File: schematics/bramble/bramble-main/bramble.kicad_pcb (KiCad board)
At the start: 2 copper layers, 50.4 x 70.6 mm, 78 parts, among them IC1 RP2040_QFN56, J1 Conn_01x05_Pin, J2 Conn_01x03_Pin, J3 Conn_01x03, J4 USB_C_Receptacle_USB2.0_16P, J5 U.FL, J6 Conn_02x06_Odd_Even, Q1 DMN3300U, Q2 FDN360P, SW1 STM_RESET, SW2 BOOT, SW3 RESET, U1 Opamp_Quad, U2 STM32L031F6P6TR, U3 MCP1700x-120xxMB, U4 RFM95W-915S2, U5 W25Q16JVSS, U6 MT25QL01GBBB8ESF-0SIT, Y1 Crystal, Y2 Crystal

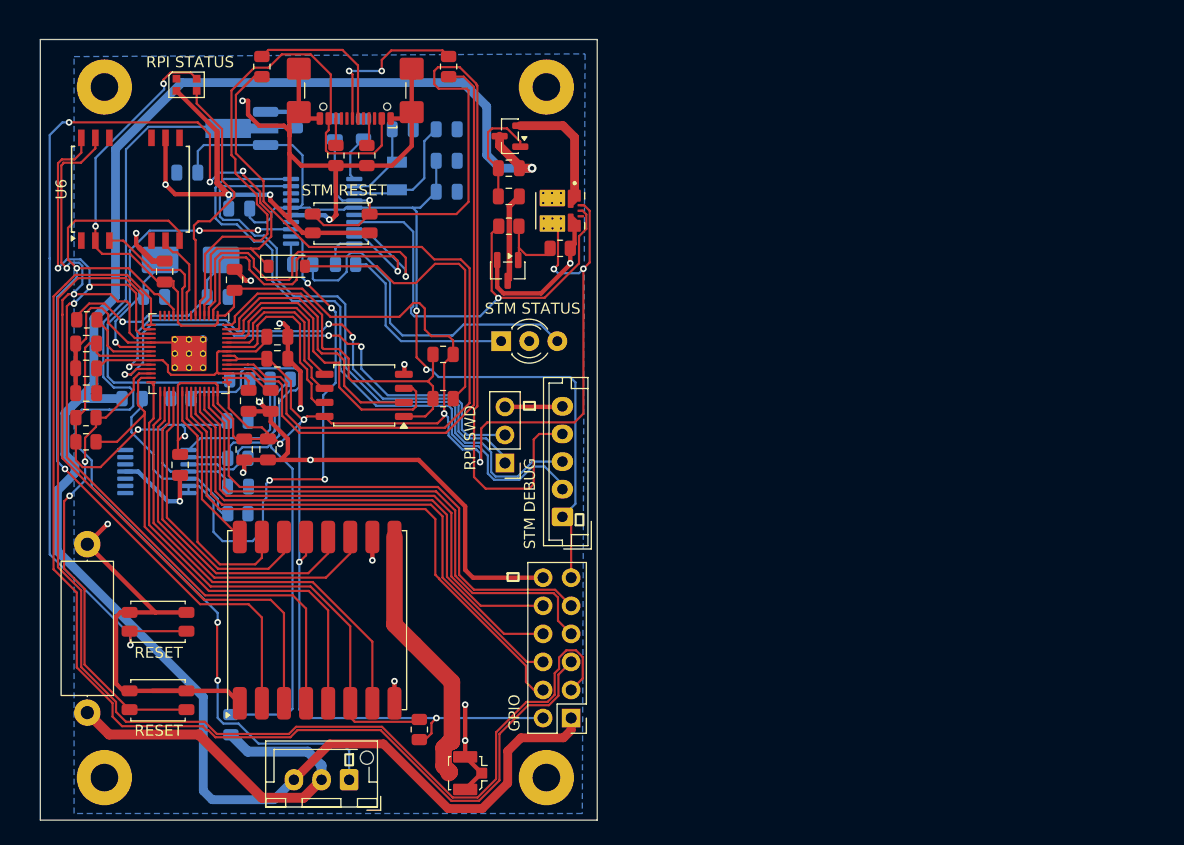
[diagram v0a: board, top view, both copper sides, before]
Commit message: Checking in v4 schematic/board prior to attempting jlcpcb run
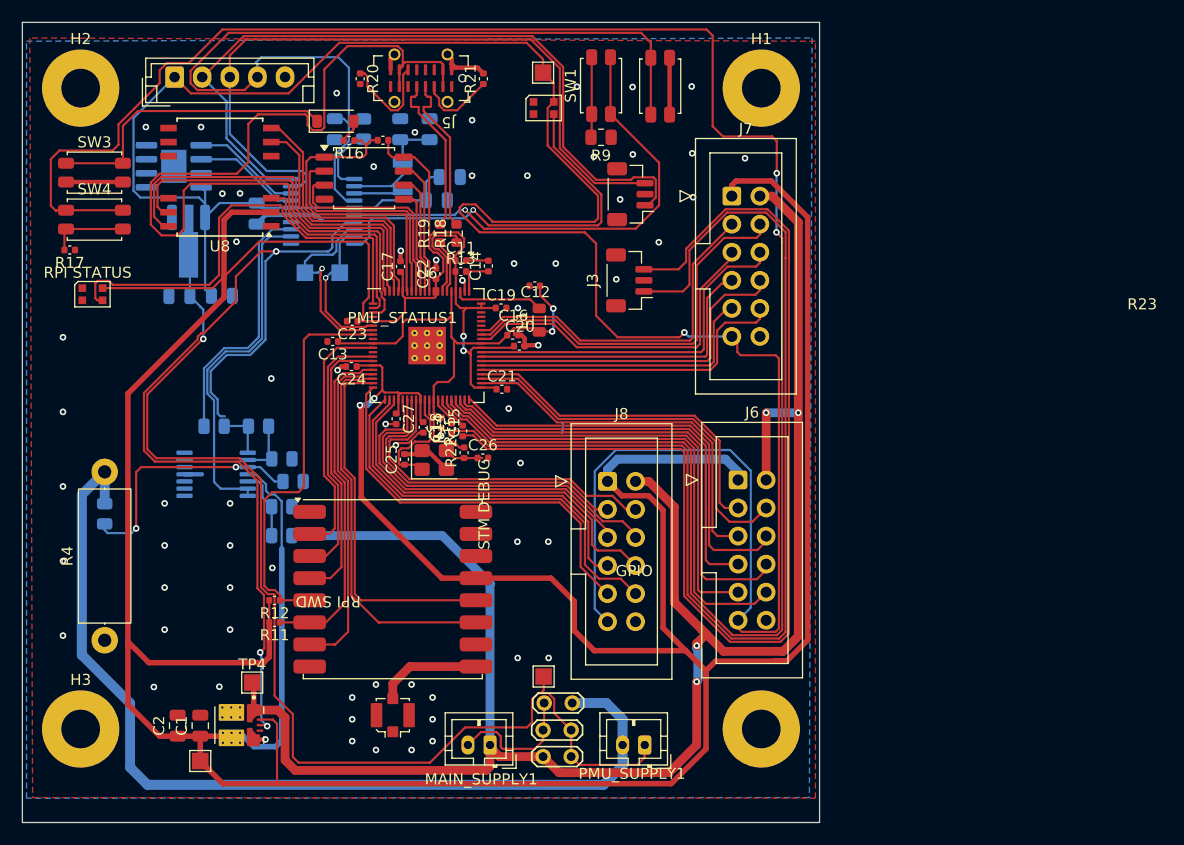
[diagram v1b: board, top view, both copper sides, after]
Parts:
- removed the C10 at (21.2, 36.0)
- removed the C9 at (15.1, 42.5)
- removed the D1 at (52.7, 40.0)
- removed IC1: RP2040_QFN56, RP2040:RP2040-QFN-56
- removed Q1: DMN3300U, Package_TO_SOT_SMD:SOT-23
- removed Q2: FDN360P, Package_TO_SOT_SMD:SOT-23
- removed R24: 5.1K, Resistor_SMD:R_0805_2012Metric
- removed R25: 10K, Resistor_SMD:R_0805_2012Metric
- removed the R5 at (28.2, 74.7)
- removed the R6 at (23.7, 45.2)
- removed the R7 at (28.8, 50.6)
- removed the R8 at (15.2, 58.4)
- removed the SW2 at (21.6, 65.4)
- removed TPS_C_IN1: 10uF, Capacitor_SMD:C_0805_2012Metric
- removed TPS_C_OUT1: 22uF, Capacitor_SMD:C_0805_2012Metric
- removed U$1, U$2, U$3, U$4: MOUNTINGHOLE2.5, MountingHole:MountingHole_2.5mm_Pad
- added C1: 10uF, Capacitor_SMD:C_0805_2012Metric, F.Cu at (25.4, 74.8)
- added C2: 22uF, Capacitor_SMD:C_0805_2012Metric, F.Cu at (23.4, 74.8)
- added C23: 100n, Capacitor_SMD:C_0402_1005Metric, F.Cu at (39.2, 38.2)
- added C24: 100n, Capacitor_SMD:C_0402_1005Metric, F.Cu at (39.1, 42.3)
- added C25: 15p, Capacitor_SMD:C_0402_1005Metric, F.Cu at (43.9, 50.7)
- added C26: 15p, Capacitor_SMD:C_0402_1005Metric, F.Cu at (51.0, 50.6)
- added C27: 100n, Capacitor_SMD:C_0402_1005Metric, F.Cu at (43.1, 47.0)
- added H1: MountingHole, MountingHole:MountingHole_3.5mm_Pad, F.Cu at (76.2, 17.1)
- added H2: MountingHole, MountingHole:MountingHole_3.5mm_Pad, F.Cu at (14.6, 17.1)
- added H3: MountingHole, MountingHole:MountingHole_3.5mm_Pad, F.Cu at (14.6, 75.1)
- added H4: MountingHole, MountingHole:MountingHole_3.5mm_Pad, F.Cu at (76.2, 75.1)
- added J7: GPIO2, Connector_IDC:IDC-Header_2x06_P2.54mm_Vertical, F.Cu at (73.5, 26.9)
- added J8: GPIO3, Connector_IDC:IDC-Header_2x06_P2.54mm_Vertical, F.Cu at (62.3, 52.7)
- added JP1: Series, TestPoint:TestPoint_2Pads_Pitch2.54mm_Drill0.8mm, F.Cu at (56.5, 75.2)
- added JP2: Parallel 1, TestPoint:TestPoint_2Pads_Pitch2.54mm_Drill0.8mm, F.Cu at (56.5, 77.6)
- added JP3: Parallel 2, TestPoint:TestPoint_2Pads_Pitch2.54mm_Drill0.8mm, F.Cu at (56.5, 72.8)
- added L1: 3.3, Inductor_SMD:L_0805_2012Metric, F.Cu at (56.1, 38.1)
- added MAIN_SUPPLY1: ~, Connector_JST:JST_PH_B2B-PH-K_1x02_P2.00mm_Vertical, F.Cu at (51.6, 76.5)
- added PMU_STATUS1: WS2812B-2020, LED_SMD:LED_WS2812B-2020_PLCC4_2.0x2.0mm, F.Cu at (56.5, 18.9)
- added PMU_SUPPLY1: ~, Connector_JST:JST_PH_B2B-PH-K_1x02_P2.00mm_Vertical, F.Cu at (65.7, 76.5)
- added R11: 10k, Capacitor_SMD:C_0402_1005Metric, F.Cu at (32.1, 65.5)
- added R12: 10k, Capacitor_SMD:C_0402_1005Metric, F.Cu at (32.1, 63.5)
- added R15: 100, Capacitor_SMD:C_0402_1005Metric, F.Cu at (49.2, 48.1)
- added R9: 10k, Resistor_SMD:R_0805_2012Metric, F.Cu at (61.7, 21.6)
- added SW1: STM_WAKE, Button_Switch_SMD:SW_SPST_EVQP2_MiddlePushTravel_H2.5mm, F.Cu at (61.7, 16.9)
- added SW4: RESET, Button_Switch_SMD:SW_SPST_EVQP2_MiddlePushTravel_H2.5mm, F.Cu at (15.8, 29.0)
- added TP1: 3V3 TEST, TestPoint:TestPoint_Pad_1.5x1.5mm, F.Cu at (25.4, 78.0)
- added TP2: RX_TEST, TestPoint:TestPoint_Pad_1.5x1.5mm, B.Cu at (38.0, 33.8)
- added TP3: TX_TEST, TestPoint:TestPoint_Pad_1.5x1.5mm, B.Cu at (34.9, 33.8)
- added TP4: MAINS TEST, TestPoint:TestPoint_Pad_1.5x1.5mm, F.Cu at (30.1, 70.9)
- added TP5: TAP TEST, TestPoint:TestPoint_Pad_1.5x1.5mm, F.Cu at (56.5, 70.3)
- added TP6: PMU SUPPLY TEST, TestPoint:TestPoint_Pad_1.5x1.5mm, F.Cu at (56.5, 15.7)
- added U4: FM24CL16B-GTR, Package_SO:SOIC-8-1EP_3.9x4.9mm_P1.27mm_EP2.29x3mm, B.Cu at (23.0, 24.2)
- added U6: RP2350_80QFN, RP2350_80QFN_minimal:RP2350-QFN-80-1EP_10x10_P0.4mm_EP3.4x3.4mm_ThermalVias, F.Cu at (46.0, 40.4)
- C11: value 8pF -> 4.7uF; footprint Capacitor_SMD:C_0805_2012Metric -> Capacitor_SMD:C_0402_1005Metric; moved to F.Cu
- C12: value 1uF -> 4.7uF; footprint Capacitor_SMD:C_0805_2012Metric -> Capacitor_SMD:C_0402_1005Metric
- C13, C17, C19, C20, C21: value 0.1uF -> 100n; footprint Capacitor_SMD:C_0805_2012Metric -> Capacitor_SMD:C_0402_1005Metric
- C14: value 0.1uF -> 4.7u; footprint Capacitor_SMD:C_0805_2012Metric -> Capacitor_SMD:C_0402_1005Metric
- C15: value 1uF -> 4.7u; footprint Capacitor_SMD:C_0805_2012Metric -> Capacitor_SMD:C_0402_1005Metric
- C16, C18, C22: value 1uF -> 100n; footprint Capacitor_SMD:C_0805_2012Metric -> Capacitor_SMD:C_0402_1005Metric
- J2: value Conn_01x03_Pin -> UART; footprint Connector_JST:JST_XH_B3B-XH-AM_1x03_P2.50mm_Vertical -> Connector_JST:JST_SH_BM03B-SRSS-TB_1x03-1MP_P1.00mm_Vertical
- J3: value Conn_01x03 -> RPI SWD; footprint Connector_PinHeader_2.54mm:PinHeader_1x03_P2.54mm_Vertical -> Connector_JST:JST_SH_BM03B-SRSS-TB_1x03-1MP_P1.00mm_Vertical
- J5: renamed from J4; footprint Connector_USB:USB_C_Receptacle_GCT_USB4110 -> Connector_USB:USB_C_Receptacle_G-Switch_GT-USB-7051x
- J6: value Conn_02x06_Odd_Even -> GPIO1; footprint Connector_PinHeader_2.54mm:PinHeader_2x06_P2.54mm_Vertical -> Connector_IDC:IDC-Header_2x06_P2.54mm_Vertical
- R1: value 100 -> 1k; moved to B.Cu
- R13: value 150 -> 33; footprint Resistor_SMD:R_0805_2012Metric -> Capacitor_SMD:C_0402_1005Metric; moved to F.Cu
- R14: value 150 -> 100; footprint Resistor_SMD:R_0805_2012Metric -> Capacitor_SMD:C_0402_1005Metric; moved to F.Cu
- R16: value 10K -> 1K; footprint Resistor_SMD:R_0805_2012Metric -> Capacitor_SMD:C_0402_1005Metric
- R17: value 1k -> 1K; footprint Resistor_SMD:R_0805_2012Metric -> Capacitor_SMD:C_0402_1005Metric
- R18: value 1K -> 27; footprint Resistor_SMD:R_0805_2012Metric -> Resistor_SMD:R_0603_1608Metric
- R19: value 10K -> 27; footprint Resistor_SMD:R_0805_2012Metric -> Resistor_SMD:R_0603_1608Metric
- R2: value 10k -> 100; moved to B.Cu
- R20: value 10K -> 5.1K; footprint Resistor_SMD:R_0805_2012Metric -> Capacitor_SMD:C_0402_1005Metric
- R21, R22: value 22 ohm -> 1K; footprint Resistor_SMD:R_0805_2012Metric -> Capacitor_SMD:C_0402_1005Metric
- R23: value 5.1K -> 10K; footprint Resistor_SMD:R_0805_2012Metric -> Capacitor_SMD:C_0402_1005Metric
- R3: value 100k -> 1k; footprint Capacitor_SMD:C_0805_2012Metric -> Resistor_SMD:R_0805_2012Metric; moved to B.Cu
- R4: value 10k -> 0.1; footprint Capacitor_SMD:C_0805_2012Metric -> Resistor_THT:R_Axial_DIN0414_L11.9mm_D4.5mm_P15.24mm_Horizontal
- SW3: value RESET -> BOOT
- Y2: value Crystal -> ABM8-272-T3; footprint Crystal:Crystal_SMD_Abracon_ABM3-2Pin_5.0x3.2mm_HandSoldering -> Crystal:Crystal_SMD_3225-4Pin_3.2x2.5mm; moved to F.Cu
- moved J2 58.8 mm to (64.3, 26.7), turned to 90 degrees
- moved R4 56.2 mm to (16.8, 67.1), turned to 90 degrees
- moved VR1 54.9 mm to (28.9, 74.8)
- moved J1 53.1 mm to (23.1, 16.1), turned to 0 degrees
- moved SW3 48.1 mm to (15.8, 24.8), turned to 0 degrees
- moved R19 44.9 mm to (47.1, 30.3), turned to 90 degrees
- moved R1 44.9 mm to (16.8, 55.6), turned to 90 degrees
- moved C12 41.7 mm to (55.7, 35.0)
- moved R20 41.2 mm to (39.9, 16.2), turned to -90 degrees
- moved C16 38.6 mm to (53.7, 39.5), turned to 0 degrees
- moved R22 35.0 mm to (49.3, 50.1), turned to 90 degrees
- moved R16 34.6 mm to (38.9, 21.8), turned to 180 degrees
- moved C20 32.8 mm to (54.3, 40.5), turned to 0 degrees
- moved R2 32.1 mm to (33.8, 52.7)
- moved SW2 31.4 mm to (67.0, 16.9), turned to 90 degrees
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- renumbered C8 to C10, C1 to C3, C2 to C4, C3 to C5, C4 to C6, C5 to C7, C6 to C8, C7 to C9, D2 to D1, J5 to J4, R15 to R10, R9 to R5, R10 to R6, R11 to R7, R12 to R8, SW1 to SW2, U4 to U5, U5 to U7, U6 to U8
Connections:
- C10 pad 1: Net-(U2-PC15-OSC32_OUT) -> Net-(U2-PC14-OSC32_IN)
- C11 pad 1: GND -> +3V3
- C11 pad 2: Net-(C11-Pad2) -> GND
- C12 pad 1: 1.2V -> +1V1
- C13 pad 1: GND -> +1V1
- C13 pad 2: 1.2V -> GND
- C14 pad 1: GND -> /rp2350B (page 4)/VREG_AVDD
- C14 pad 2: 1.2V -> GND
- C15 pad 1: +3V3 -> +1V1
- C16 pad 1: +3V3 -> +1V1
- C6 pad 2: Net-(J2-Pin_1) -> Net-(JP1-B)
- D1 pad 1: /rp2040/USBBOOT -> /rp2350B (page 4)/USBBOOT
- D1 pad 2: Net-(D2-A) -> Net-(D1-A)
- J2 pad 1: Net-(J2-Pin_1) -> Net-(J1-Pin_2)
- J2 pad 2: GNDPWR -> GND
- J2 pad 3: +9V -> Net-(J1-Pin_3)
- J3 pad 1: /rp2040/SWCLK -> Net-(J3-Pin_1)
- J3 pad 2: /rp2040/SWDIO -> GND
- J3 pad 3: GND -> Net-(J3-Pin_3)
- J5 pad A5: Net-(J4-CC1) -> Net-(J5-CC1)
- J5 pad A6: Net-(J4-D+-PadA6) -> /rp2350B (page 4)/D+
- J5 pad A7: Net-(J4-D--PadA7) -> /rp2350B (page 4)/D-
- J5 pad B5: Net-(J4-CC2) -> Net-(J5-CC2)
- J6 pad 1: +9V -> +3V3
- J6 pad 10: /rp2040/MOTOR_LO_2 -> /rp2350B (page 4)/MOTOR_HI_1
- J6 pad 2: +3V3 -> +9V
- J6 pad 3: /rp2040/VALVE_3 -> /rp2350B (page 4)/VALVE_3
- J6 pad 4: /rp2040/MOTOR_HI_1 -> /rp2350B (page 4)/MOTOR_LO_2
- J6 pad 5: /rp2040/VALVE_4 -> /rp2350B (page 4)/VALVE_4
- J6 pad 6: /rp2040/MOTOR_HI_2 -> /rp2350B (page 4)/MOTOR_LO_1
- J6 pad 7: /rp2040/VALVE_2 -> /rp2350B (page 4)/VALVE_2
- J6 pad 8: /rp2040/MOTOR_LO_1 -> /rp2350B (page 4)/MOTOR_HI_2
- J6 pad 9: /rp2040/VALVE_1 -> /rp2350B (page 4)/VALVE_1
- R1 pad 1: Net-(Q1-G) -> Net-(U1A-+)
- R1 pad 2: /pmu/3V3_POWER_ON -> GNDPWR
- R13 pad 1: Net-(D1-A1) -> +3V3
- R13 pad 2: Net-(U2-PA4) -> /rp2350B (page 4)/VREG_AVDD
- R14 pad 1: Net-(D1-A2) -> Net-(J3-Pin_1)
- R14 pad 2: Net-(U2-PA5) -> Net-(U6-SWCLK)
- R16 pad 1: +3V3 -> /rp2350B (page 4)/QSPI_SS
- R16 pad 2: /rp2040/~{RESET} -> Net-(D1-A)
- R17 pad 1: Net-(C11-Pad2) -> GND
- R18 pad 1: /rp2040/QSPI_CS -> Net-(U6-USB_DP)
- R18 pad 2: Net-(D2-A) -> /rp2350B (page 4)/D+
- R19 pad 1: /rp2040/RFM_RST -> Net-(U6-USB_DM)
- R19 pad 2: +3V3 -> /rp2350B (page 4)/D-
- R2 pad 1: Net-(Q1-G) -> Net-(U1A-+)
- R20 pad 1: /rp2040/RFM_CS -> Net-(J5-CC2)
- R20 pad 2: +3V3 -> GND
- R21 pad 1: Net-(J4-D+-PadA6) -> Net-(J5-CC1)
- R21 pad 2: /rp2040/D- -> GND
- R22 pad 1: Net-(J4-D--PadA7) -> Net-(C26-Pad1)
- R22 pad 2: /rp2040/D+ -> /rp2350B (page 4)/XOUT
- R23 pad 1: GND -> +3V3
- R23 pad 2: Net-(J4-CC2) -> /rp2350B (page 4)/QSPI_SS
- R3 pad 1: Net-(Q2-G) -> GND
- R3 pad 2: Net-(Q1-D) -> Net-(U1A--)
- R4 pad 1: +9V -> GND
- R4 pad 2: Net-(Q2-G) -> GNDPWR
- RPI_STATUS1 pad 3: /rp2040/RGB_LED -> /rp2350B (page 4)/RGB_LED
- SW3 pad 1: /rp2040/~{RESET} -> /rp2350B (page 4)/USBBOOT
- U2 pad 10: Net-(U2-PA4) -> Net-(PMU_STATUS1-DIN)
- U2 pad 11: Net-(U2-PA5) -> unconnected-(U2-PA5-Pad11)
- U2 pad 17: unconnected-(U2-PA9-Pad17) -> /pmu/SCL
- U2 pad 18: unconnected-(U2-PA10-Pad18) -> /pmu/SDA
- U2 pad 3: Net-(U2-PC15-OSC32_OUT) -> Net-(U2-PC14-OSC32_IN)
- U2 pad 6: unconnected-(U2-PA0-CK_IN-Pad6) -> Net-(U2-PA0-CK_IN)
- U2 pad 8: /rp2040/RX -> /rp2350B (page 4)/RX
- U2 pad 9: /rp2040/TX -> /rp2350B (page 4)/TX
- U3 pad 2: Net-(J2-Pin_1) -> Net-(JP1-B)
- U5 pad 11: /rp2040/RFM_IO3 -> /rp2350B (page 4)/RFM_IO2
- U5 pad 12: /rp2040/RFM_IO4 -> /rp2350B (page 4)/RFM_IO1
- U5 pad 14: /rp2040/RFM_IO0 -> /rp2350B (page 4)/RFM_IO5
- U5 pad 15: /rp2040/RFM_IO1 -> /rp2350B (page 4)/RFM_IO4
- U5 pad 16: /rp2040/RFM_IO2 -> /rp2350B (page 4)/RFM_IO3
- U5 pad 2: /rp2040/MISO -> /rp2350B (page 4)/MISO
- U5 pad 3: /rp2040/MOSI -> /rp2350B (page 4)/MOSI
- U5 pad 4: /rp2040/SCK -> /rp2350B (page 4)/SCK
- U5 pad 5: /rp2040/RFM_CS -> /rp2350B (page 4)/RFM_CS
- U5 pad 6: /rp2040/RFM_RST -> /rp2350B (page 4)/RFM_RST
- U5 pad 7: /rp2040/RFM_IO5 -> /rp2350B (page 4)/RFM_IO0
- U7 pad 1: /rp2040/QSPI_CS -> /rp2350B (page 4)/QSPI_SS
- U7 pad 2: /rp2040/QSPI_D1 -> /rp2350B (page 4)/QSPI_D1
- U7 pad 3: /rp2040/QSPI_D2 -> /rp2350B (page 4)/QSPI_D2
- U7 pad 5: /rp2040/QSPI_D0 -> /rp2350B (page 4)/QSPI_D0
- U7 pad 6: /rp2040/QSPI_SCK -> /rp2350B (page 4)/QSPI_SCK
- U7 pad 7: /rp2040/QSPI_D3 -> /rp2350B (page 4)/QSPI_D3
- U8 pad 15: /rp2040/MOSI -> /rp2350B (page 4)/MT25_MOSI
- U8 pad 16: /rp2040/SCK -> /rp2350B (page 4)/MT25_SCK
- U8 pad 3: /rp2040/MT25_RESET -> /rp2350B (page 4)/MT25_RESET
- U8 pad 7: /rp2040/MT25_CS -> /rp2350B (page 4)/MT25_CS
- U8 pad 8: /rp2040/MISO -> /rp2350B (page 4)/MT25_MISO
- VR1 pad 1: Net-(Q2-S) -> +9V
- Y1 pad 2: Net-(U2-PC15-OSC32_OUT) -> Net-(U2-PC14-OSC32_IN)
- Y2 pad 1: Net-(C11-Pad2) -> /rp2350B (page 4)/XIN
- Y2 pad 2: Net-(IC1-XIN) -> GND
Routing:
- net GND: track 253.5 -> 43.8 mm, vias 20 -> 67
- net /rp2350B (page 4)/RUN: track 0.00 -> 184.1 mm, vias 0 -> 2
- net +3V3: track 277.4 -> 424.4 mm, vias 12 -> 4
- net VDD: track 88.3 -> 231.9 mm, vias 2 -> 1
- net /rp2040/VALVE_3: track 111.8 -> 0.00 mm
- net Net-(JP1-B): track 0.00 -> 108.0 mm, vias 0 -> 1
- net /rp2040/VALVE_4: track 107.1 -> 0.00 mm
- net Net-(J3-Pin_1): track 0.00 -> 100.5 mm
- net /rp2040/USBBOOT: track 99.9 -> 0.00 mm, vias 4 -> 0
- net Net-(J3-Pin_3): track 0.00 -> 98.5 mm
- net Net-(J2-Pin_1): track 96.3 -> 0.00 mm, vias 2 -> 0
- net /rp2040/SCK: track 80.4 -> 0.00 mm, vias 3 -> 0
- net /rp2040/MOSI: track 78.7 -> 0.00 mm, vias 2 -> 0
- net /rp2040/MISO: track 76.8 -> 0.00 mm, vias 2 -> 0
- net /rp2040/D-: track 73.9 -> 0.00 mm
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- added copper zone on F.Cu, net GND
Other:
- board size 50.4 x 70.6 mm -> 72.1 x 72.4 mm
- board text added: "v0.4, March 2026 E. E. Beerepoot"
- board text removed: "PWR"
- board text removed: "RESET"
- board text removed: "RPI_SWD"
- board text removed: "STM RESET"
- board text removed: "STM STATUS"
- board text removed: "v0.4, Dec 2025 E. E. Beerepoot"
- board text removed: "⏚"
